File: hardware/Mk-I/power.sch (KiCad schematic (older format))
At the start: 14 parts, among them CON1 10118194-0001LF, U2 MCP73831T-2ACI/OT, U3 BD33IA5MEFJ-ME2

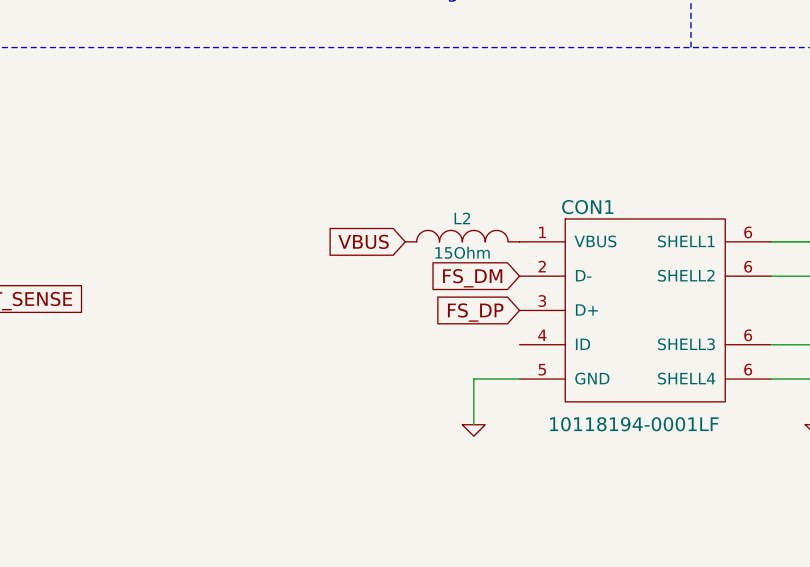
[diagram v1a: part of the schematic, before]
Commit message: HW: Finish rev-D layout
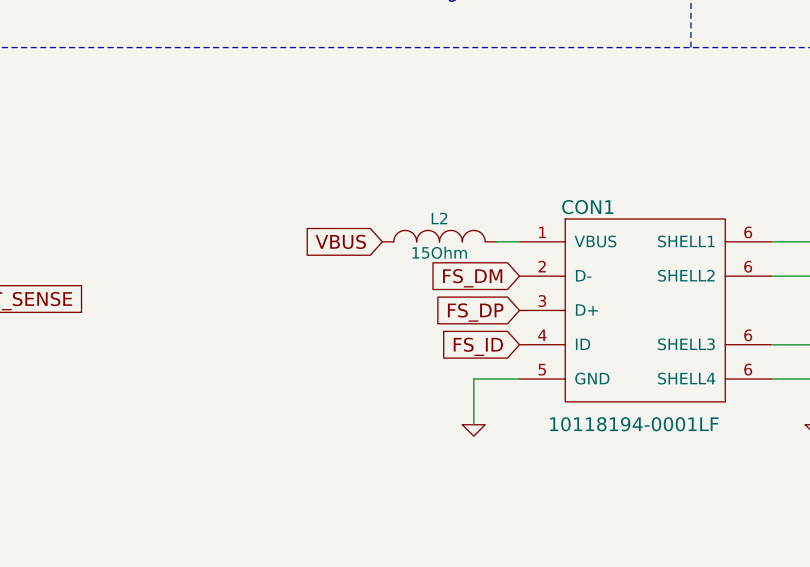
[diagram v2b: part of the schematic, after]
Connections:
- net FS_ID: now reaches CON1.4 (ID)
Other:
- moved on the sheet: L2
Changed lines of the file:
@@
 	1    0    0    -1
 $EndComp
-Text GLabel 4700 4150 0    60   Input ~ 0
+Text GLabel 4600 4150 0    60   Input ~ 0
 VBUS
 Wire Wire Line
@@
 L INDUCTOR_SMALL L2
 U 1 1 58628564
-P 4950 4150
-F 0 "L2" H 4950 4250 50  0000 C CNN
-F 1 "15Ohm" H 4950 4100 50  0000 C CNN
-F 2 "Capacitors_SMD:C_0805" H 4950 4150 60  0001 C CNN
-F 3 "" H 4950 4150 60  0000 C CNN
-	1    4950 4150
+P 4850 4150
+F 0 "L2" H 4850 4250 50  0000 C CNN
+F 1 "15Ohm" H 4850 4100 50  0000 C CNN
+F 2 "Capacitors_SMD:C_0805" H 4850 4150 60  0001 C CNN
+F 3 "" H 4850 4150 60  0000 C CNN
+	1    4850 4150
 	1    0    0    -1
 $EndComp
@@
 Text GLabel 2650 4400 2    60   Input ~ 0
 VBAT_SENSE
+Wire Wire Line
+	5200 4150 5100 4150
+Text GLabel 5200 4600 0    60   Input ~ 0
+FS_ID
 $EndSCHEMATC
